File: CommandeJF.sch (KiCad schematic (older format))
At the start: 14 parts, among them J1 Conn_01x02, J2 Conn_01x02, J3 Conn_01x04, K1 RelaisSRD, T1 Trou, T2 Trou, T3 Trou, T4 Trou, U101 MP1584, U2 DS3231

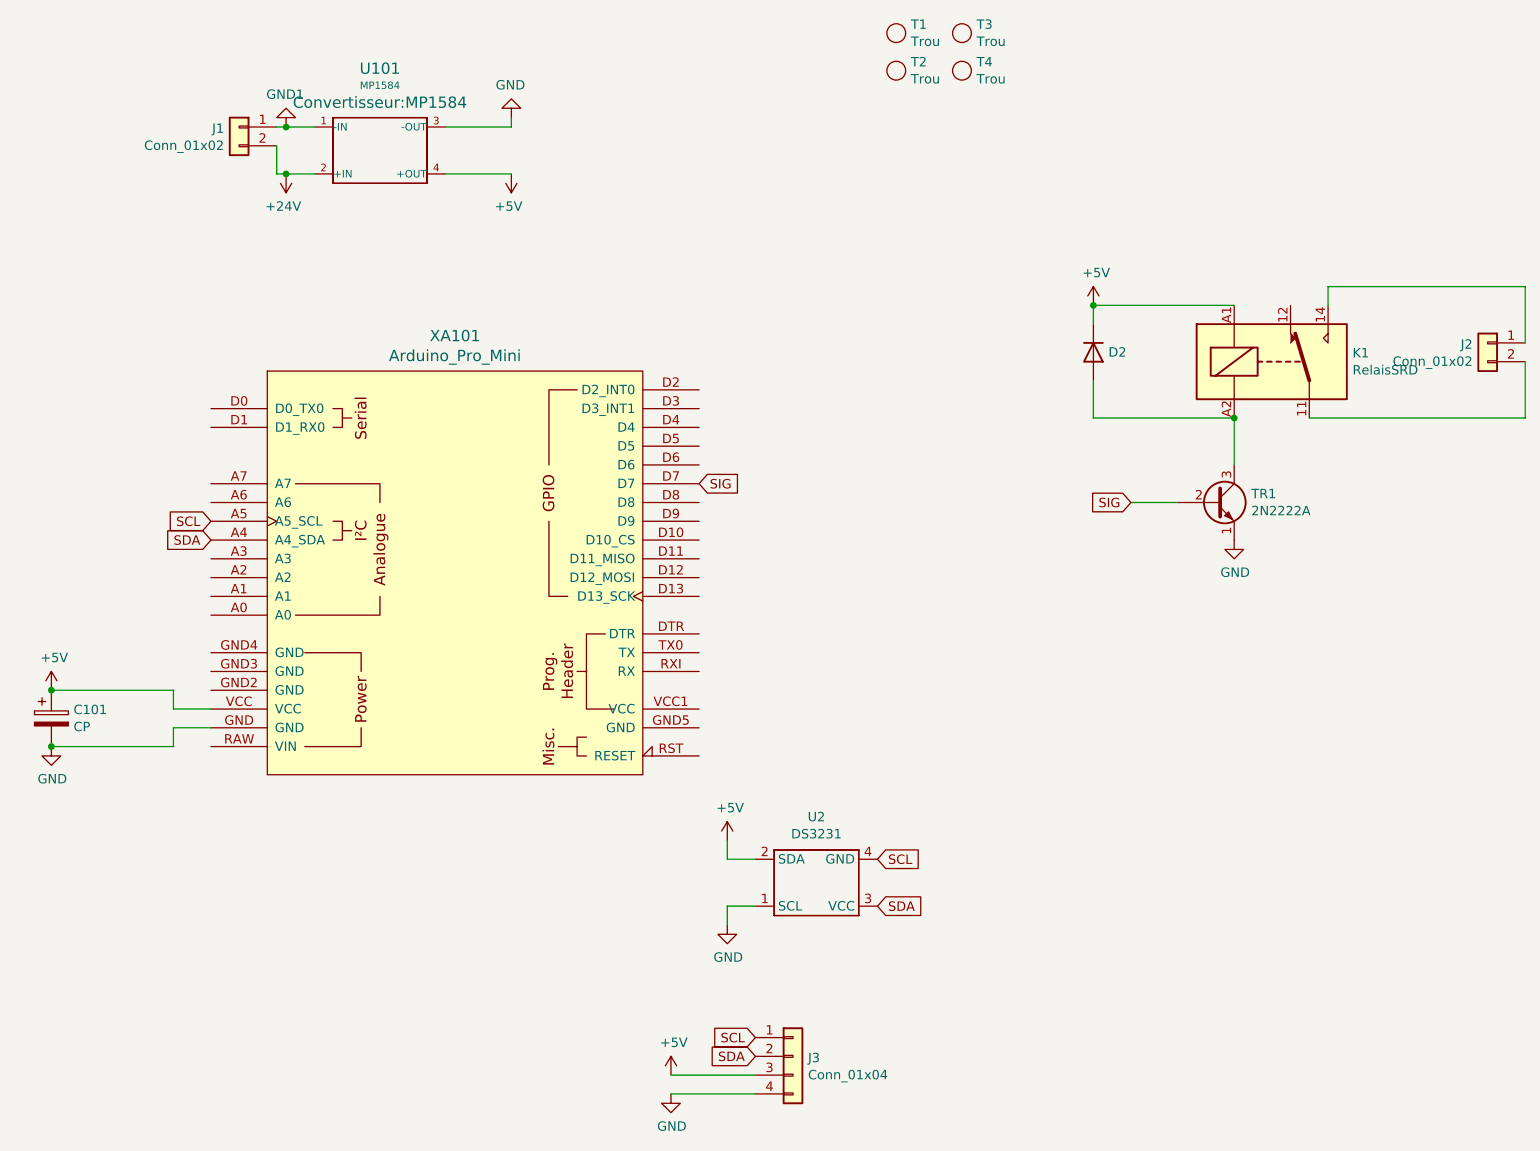
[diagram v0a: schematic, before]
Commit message: Arduino nano
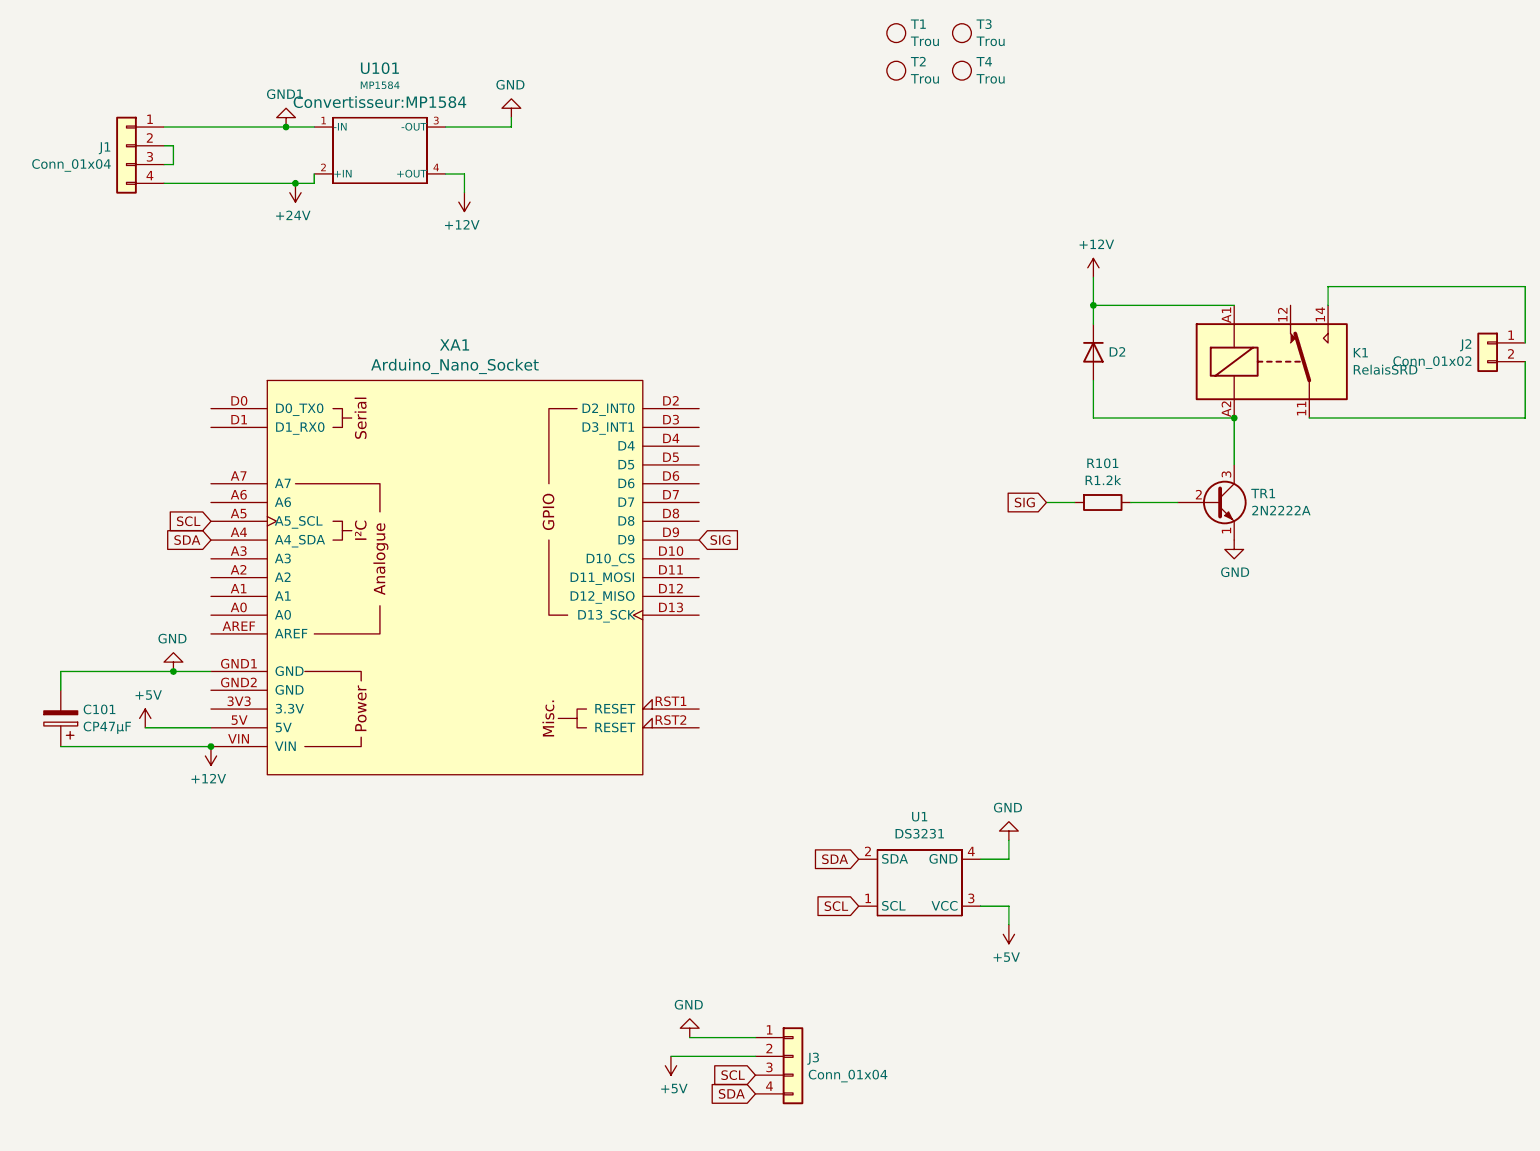
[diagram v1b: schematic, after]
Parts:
- removed J1: Conn_01x02, TerminalBlock_Phoenix:TerminalBlock_Phoenix_MKDS-1,5-2-5.08_1x02_P5.08mm_Horizontal, symbol Connector_Generic:Conn_01x02
- removed U2: DS3231, Timer_RTC:RTC_DS3231, symbol Timer_RTC:DS3231
- removed XA101: Arduino_Pro_Mini, Arduino:Arduino_Pro_Mini, symbol Arduino:Arduino_Pro_Mini
- added J1: Conn_01x04, TerminalBlock_Phoenix:TerminalBlock_Phoenix_MKDS-1,5-4-5.08_1x04_P5.08mm_Horizontal, symbol Connector_Generic:Conn_01x04
- added R101: R1.2k, Resistance:R_025W, symbol Personnel:R
- added U1: DS3231, Timer_RTC:RTC_DS3231, symbol Timer_RTC:DS3231
- added XA1: Arduino_Nano_Socket, Arduino:Arduino_Nano_Module_sur_Socket, symbol Arduino:Arduino_Nano_Socket
- C101: value CP -> CP47µF; footprint capacitors:CP_5x11mm -> capacitors:CP_5x11mm_hor
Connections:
- net +24V: now also J1.4 (Pin_4)
- net +5V: now also J3.2 (Pin_2), U1.3 (VCC), XA1.5V; no longer C101.1, D2.1 (K), J3.3 (Pin_3), K1.A1, U101.4 (+OUT)
- net GND: now also J3.1 (Pin_1), U1.4 (GND), XA1.GND1 (GND); no longer J3.4 (Pin_4)
- net GND1: now also J1.1 (Pin_1)
- net SCL: now also J3.3 (Pin_3), U1.1 (SCL), XA1.A5 (A5_SCL); no longer J3.1 (Pin_1)
- net SDA: now also J3.4 (Pin_4), U1.2 (SDA), XA1.A4 (A4_SDA); no longer J3.2 (Pin_2)
- net SIG: now also R101.2, XA1.D9; no longer TR1.2 (B)
- new net: R101.1, TR1.2 (B)
- new net: J1.2 (Pin_2), J1.3 (Pin_3)
- new net +12V: C101.1, D2.1 (K), K1.A1, U101.4 (+OUT), XA1.VIN
